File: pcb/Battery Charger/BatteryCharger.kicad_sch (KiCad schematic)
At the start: 11 parts, among them Q1 FS8205A, U1 DW01A, U3 MCP73831

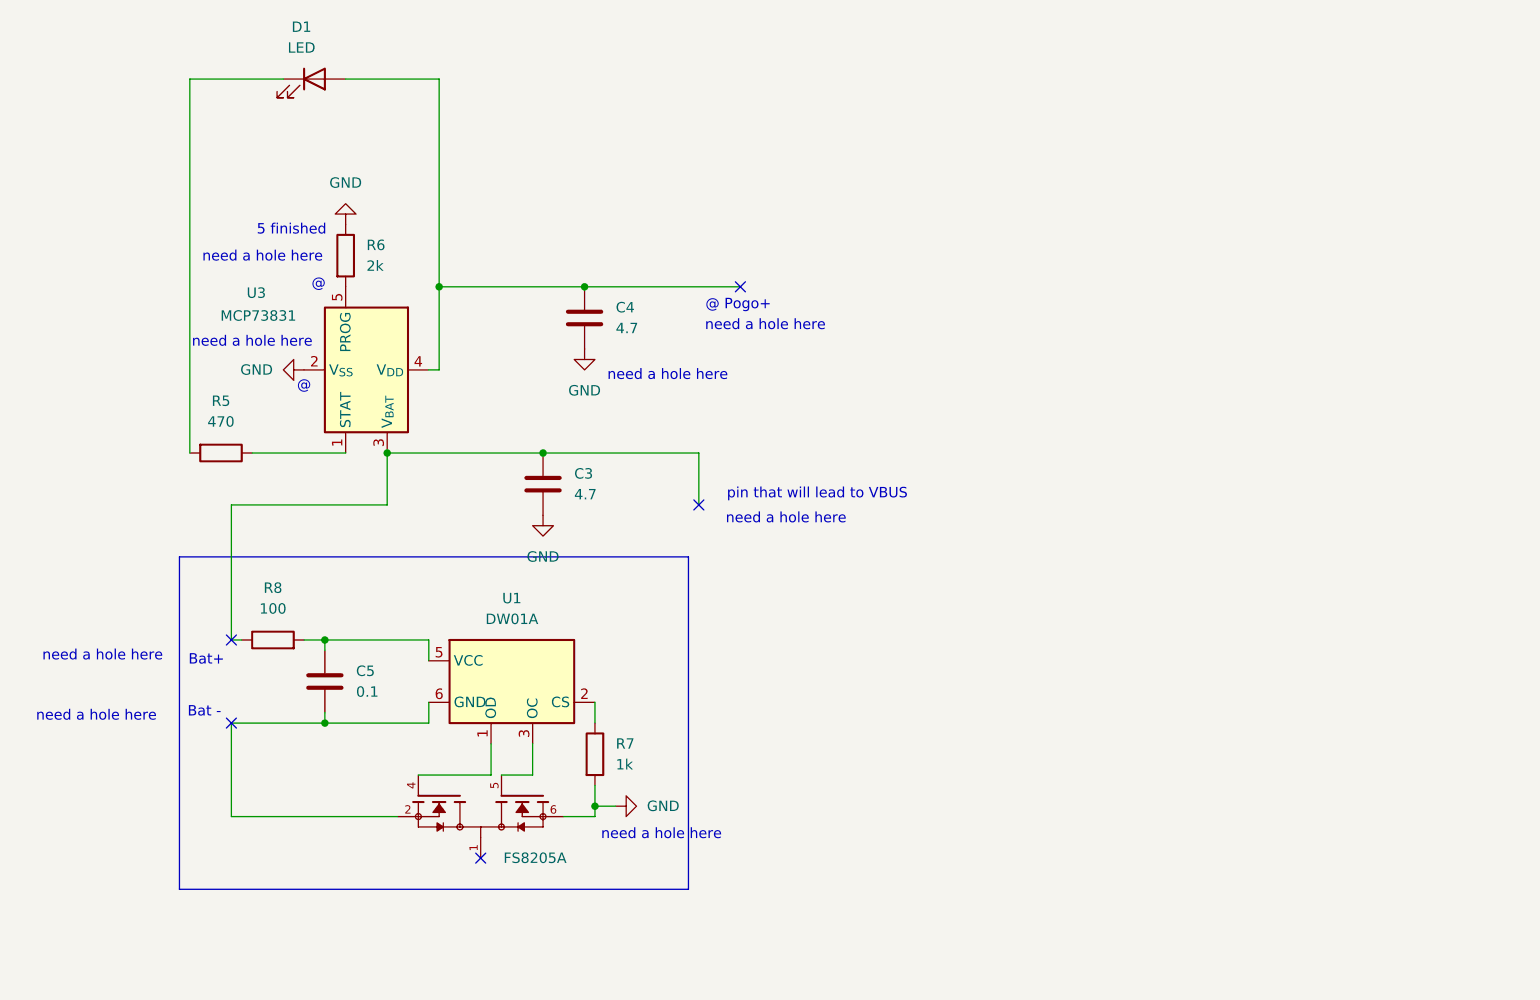
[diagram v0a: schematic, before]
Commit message: type shiii
I added the booster converter
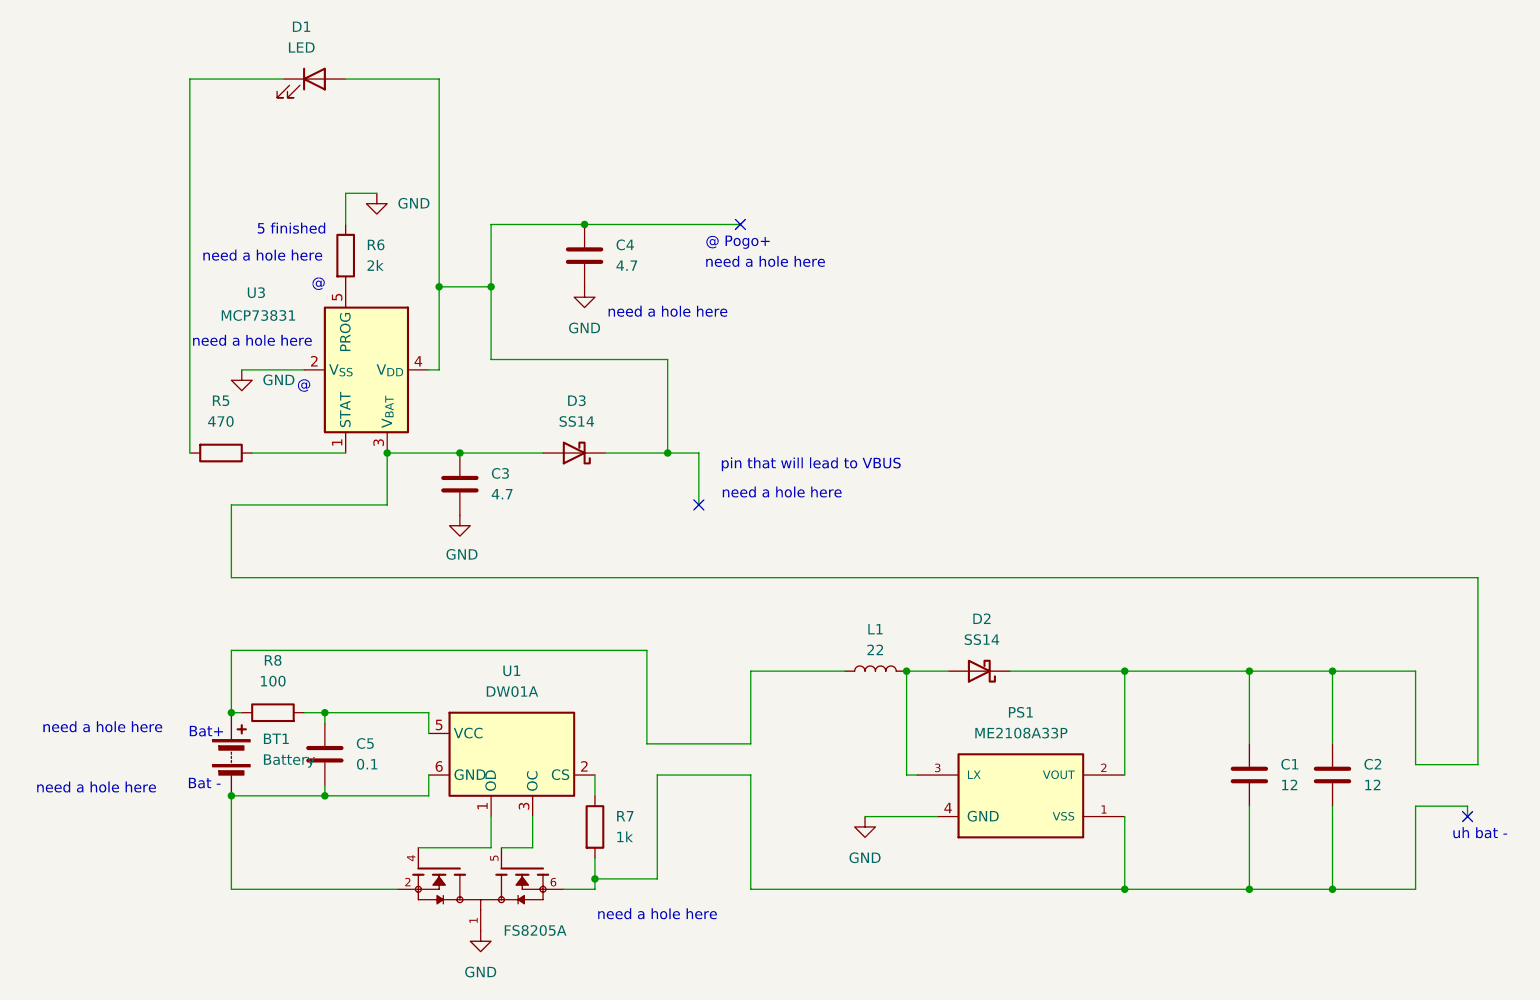
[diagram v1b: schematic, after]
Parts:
- added BT1: Battery, symbol Device:Battery
- added C1, C2: 12, symbol Device:C
- added D2, D3: SS14, Diode_SMD:D_SMA, symbol Diode:SS14
- added L1: 22, symbol Device:L
- added PS1: ME2108A33P, symbol FS8205:ME2108A33P
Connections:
- net GND: now also Q1.1, PS1.4 (GND); no longer Q1.6, Q1.7, R7.2
- net at C4.1, D1.2 (A), U3.4 (V_{DD}): now also D3.1 (K)
- net at C5.2, Q1.2, Q1.3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: now also BT1.2 (-)
- net at C3.1, U3.3 (V_{BAT}): now also C1.1, C2.1, D2.1 (K), D3.2 (A), PS1.2 (VOUT); no longer R8.1
- new net: C1.2, C2.2, PS1.1 (VSS), Q1.6, Q1.7, R7.2
- new net: D2.2 (A), L1.2, PS1.3 (LX)
- new net: BT1.1 (+), L1.1, R8.1
- no-connect marks 5 -> 3
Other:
- note added: "uh bat -"
- moved on the sheet: C3, C4, C5, R7, R8, U1
